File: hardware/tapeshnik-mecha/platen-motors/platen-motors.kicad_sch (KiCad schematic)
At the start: 5 parts, among them J1 Conn_01x03_Pin, J2 Conn_01x03_Pin, J3 Conn_01x05_Pin, J4 Conn_01x05_Pin, M1 Motor_Servo

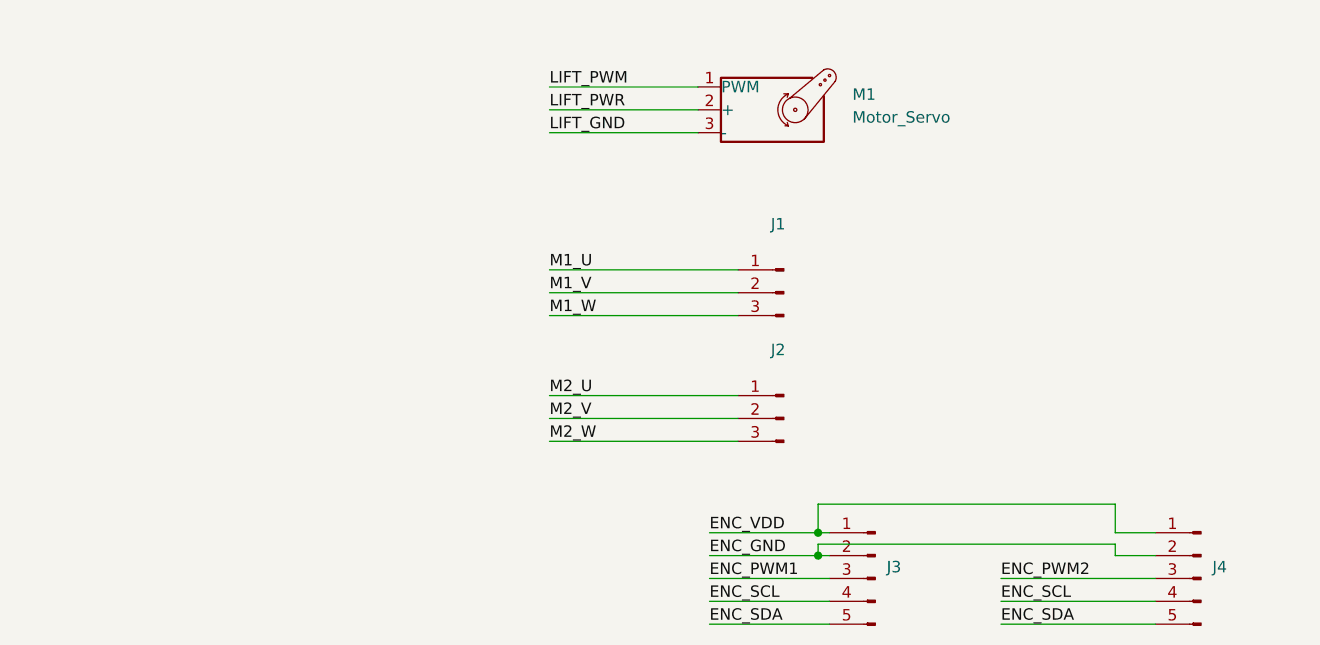
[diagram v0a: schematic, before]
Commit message: adding a lot of mecha-specific stuff
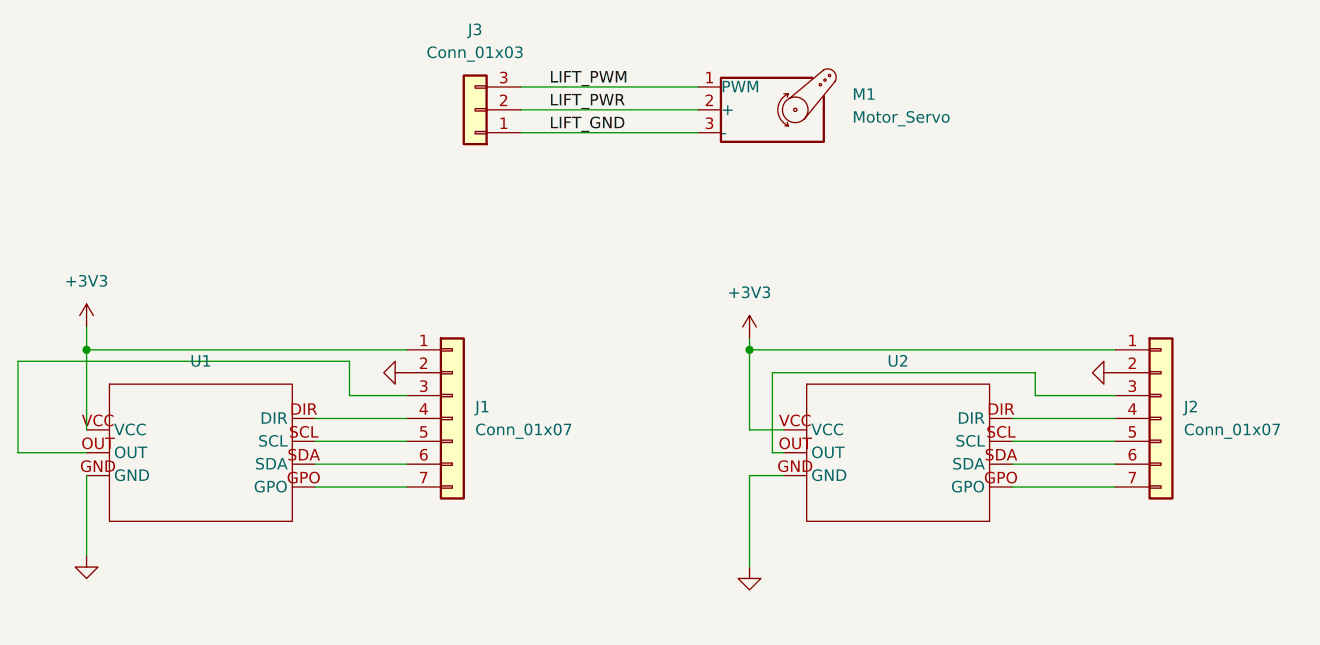
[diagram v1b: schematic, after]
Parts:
- removed J1, J2: Conn_01x03_Pin, symbol Connector:Conn_01x03_Pin
- removed J3, J4: Conn_01x05_Pin, Connector_PinHeader_2.54mm:PinHeader_1x05_P2.54mm_Vertical, symbol Connector:Conn_01x05_Pin
- added J1, J2: Conn_01x07, Connector_PinHeader_2.54mm:PinHeader_1x07_P2.54mm_Vertical, symbol Connector_Generic:Conn_01x07
- added J3: Conn_01x03, Connector_PinHeader_2.54mm:PinHeader_1x03_P2.54mm_Vertical, symbol Connector_Generic:Conn_01x03
- added U1, U2: ~, MechanicalParts:AS5600-breakout-23x23, symbol AS5600_breakout:AS5600
- M1: footprint (none) -> Connector_PinHeader_2.54mm:PinHeader_1x03_P2.54mm_Vertical
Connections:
- net LIFT_GND: now also J3.1 (Pin_1)
- net LIFT_PWM: now also J3.3 (Pin_3)
- net LIFT_PWR: now also J3.2 (Pin_2)
- new net: J1.4 (Pin_4), U1.DIR
- new net: J1.7 (Pin_7), U1.GPO
- new net: J1.3 (Pin_3), U1.OUT
- new net: J1.5 (Pin_5), U1.SCL
- new net: J1.6 (Pin_6), U1.SDA
- new net: J2.4 (Pin_4), U2.DIR
- new net: J2.7 (Pin_7), U2.GPO
- new net: J2.3 (Pin_3), U2.OUT
- new net: J2.5 (Pin_5), U2.SCL
- new net: J2.6 (Pin_6), U2.SDA
- new net +3V3: J1.1 (Pin_1), J2.1 (Pin_1), U1.VCC, U2.VCC
- new net GND: J1.2 (Pin_2), J2.2 (Pin_2), U1.GND, U2.GND
